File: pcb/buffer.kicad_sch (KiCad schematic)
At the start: 1 part

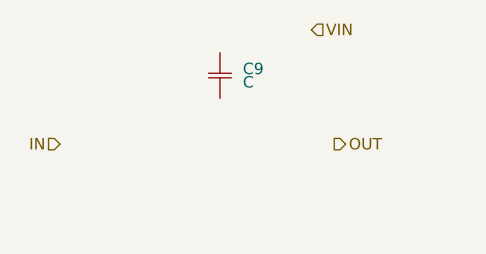
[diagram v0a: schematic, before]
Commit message: added buffer
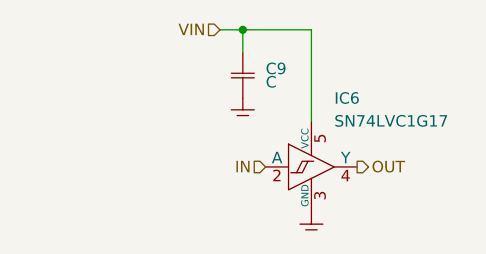
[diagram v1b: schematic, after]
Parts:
- added IC6: SN74LVC1G17, Single Schmitt-Trigger Buffer, symbol logic:SN74LVC1G17
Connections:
- net IN: now also IC6.2 (A)
- net OUT: now also IC6.4 (Y)
- net VIN: now also C9.2, IC6.5 (VCC)
- net GND: now reaches C9.1
- net GND: now also IC6.3 (GND)
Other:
- moved on the sheet: C9
